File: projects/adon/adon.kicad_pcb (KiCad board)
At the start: 2 copper layers, 56.9 x 30.1 mm, 32 parts, among them IC1 STM32F030F4, P1 BATTERY, P3 SWD, Q1 NPN2, SW1 POWER, SW2 BUTTON0, SW3 BUTTON1, SW4 BUTTON2, SW5 BUTTON3

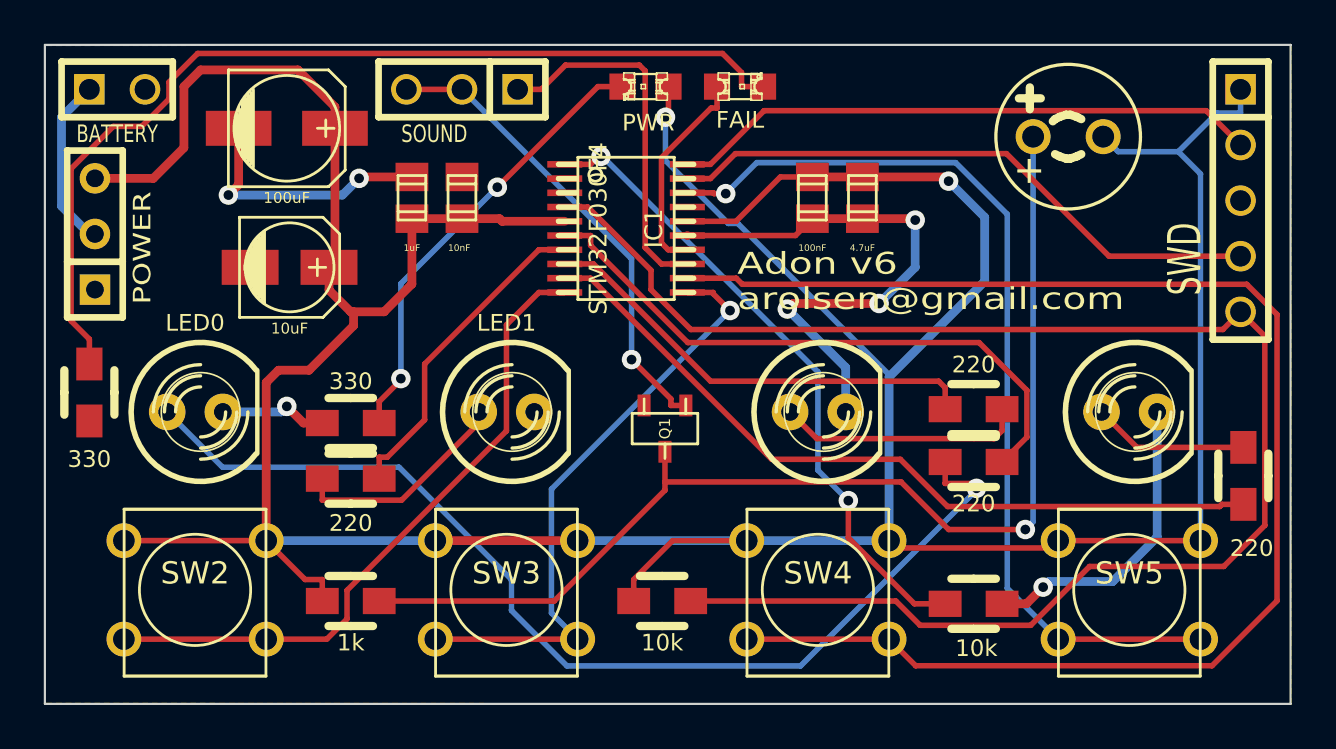
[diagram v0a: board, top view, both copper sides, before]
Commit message: totally updated, gonna be awesome
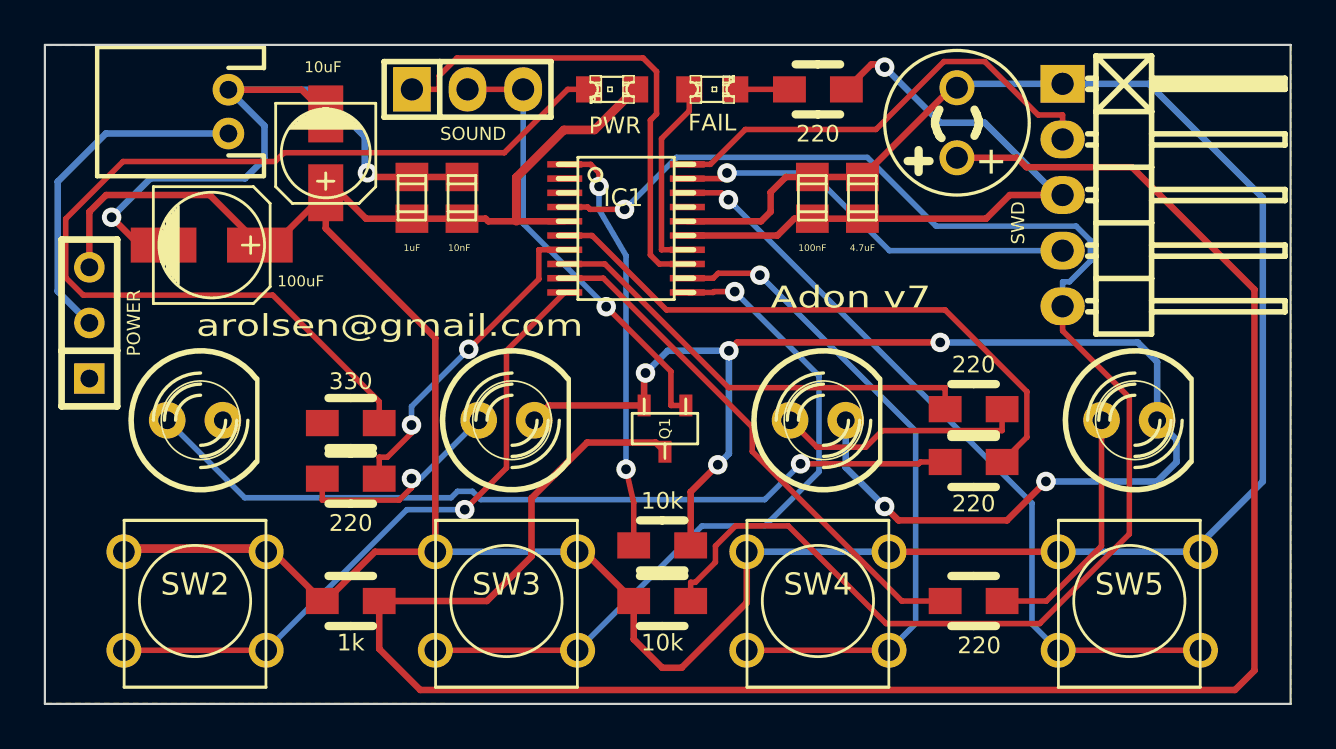
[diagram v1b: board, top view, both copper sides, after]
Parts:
- JP1: footprint synic:SIL-3 -> Pin_Headers:Pin_Header_Straight_1x03
- P1: footprint synic:SIL-2 -> jst-2-pth-ra
- P3: footprint synic:SIL-5 -> Pin_Headers:Pin_Header_Angled_1x05
- R9: value 330 -> 220
- moved R9 36.0 mm to (48.3, 15.2), turned to 0 degrees
- moved R1 14.5 mm to (41.1, 36.1)
- moved R4 13.6 mm to (55.4, 38.6), turned to 0 degrees
- moved P3 8.27 mm to (59.4, 20.1)
- moved C1 6.34 mm to (20.6, 22.4)
- moved C6 5.46 mm to (25.8, 18.2), turned to 270 degrees
- moved P1 5.18 mm to (21.3, 16.3), turned to 90 degrees
- moved SP1 5.12 mm to (54.6, 16.8), turned to 270 degrees
- moved SW1 4.07 mm to (15.0, 25.9)
- moved D1 1.53 mm to (38.9, 15.2)
- moved D6 1.28 mm to (43.4, 15.2)
- moved SW2 0.51 mm to (19.8, 38.6)
- moved SW3 0.51 mm to (34.0, 38.6)
- moved SW4 0.51 mm to (48.3, 38.6)
- moved SW5 0.51 mm to (62.5, 38.6)
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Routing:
- net GND: track 56.3 -> 128.7 mm, vias 7 -> 9
- net Net-(Q1-Pad3): track 52.4 -> 95.2 mm, vias 1 -> 0
- net Net-(D6-Pad2): track 44.5 -> 2.48 mm
- net Net-(IC1-Pad12): track 66.6 -> 30.5 mm, vias 0 -> 1
- net VDD: track 188.2 -> 161.6 mm, vias 2 -> 0
- net Net-(D1-Pad2): track 20.6 -> 46.7 mm, vias 2 -> 0
- net Net-(IC1-Pad9): track 35.4 -> 24.1 mm
- net Net-(D5-Pad1): track 48.5 -> 38.0 mm
- net Net-(IC1-Pad1): track 29.6 -> 19.1 mm
- net SWDIO: track 27.7 -> 18.7 mm, vias 0 -> 1
- net Net-(IC1-Pad18): track 43.1 -> 35.3 mm
- net Net-(P1-Pad1): track 8.29 -> 15.8 mm
- net Net-(IC1-Pad13): track 16.7 -> 22.7 mm
- net SWCLK: track 26.9 -> 21.2 mm
- net Net-(IC1-Pad11): track 27.7 -> 32.9 mm
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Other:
- board text added: "Adon v7"
- board text added: "Adon v7 arolsen@gmail.com"
- board text added: "arolsen@gmail.com"
- board text removed: "Adon v6 arolsen@gmail.com"
